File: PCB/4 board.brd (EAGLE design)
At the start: 82.6 x 57.5 mm, 17 parts, among them T1 2N2222, T2 2N2222, T3 2N2222

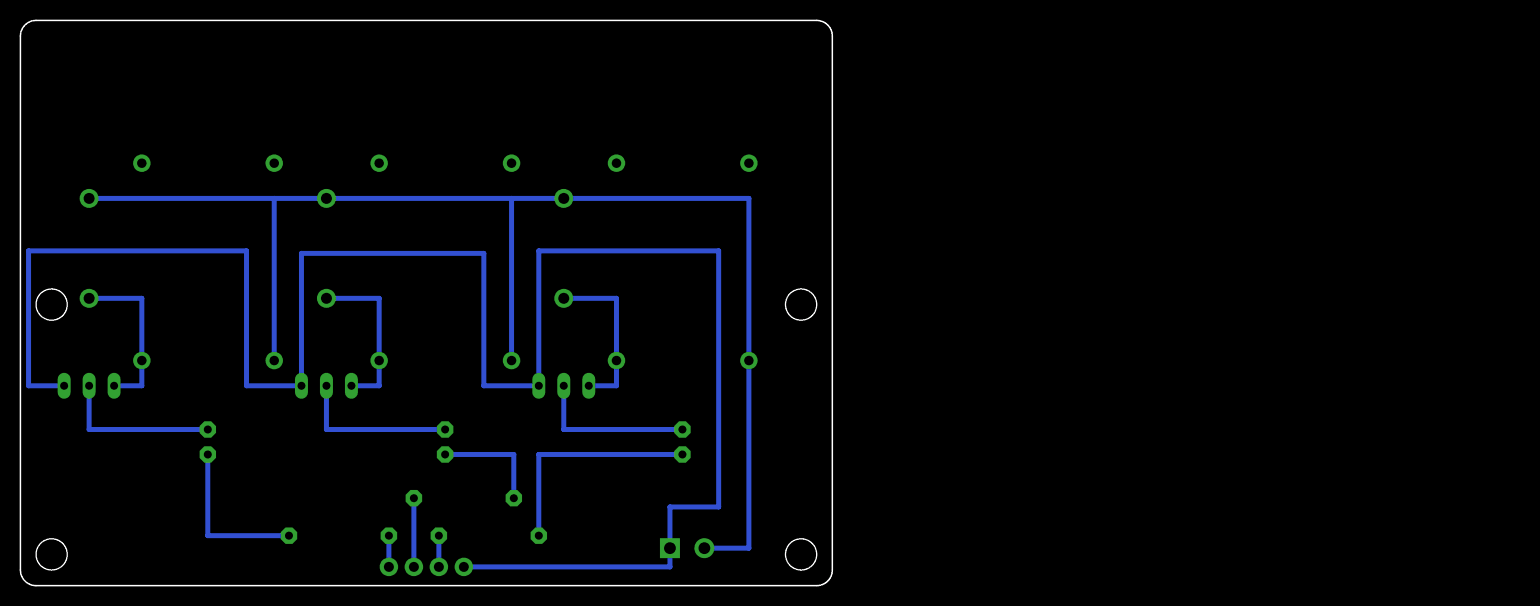
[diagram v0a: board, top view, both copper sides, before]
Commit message: 4 valve boards
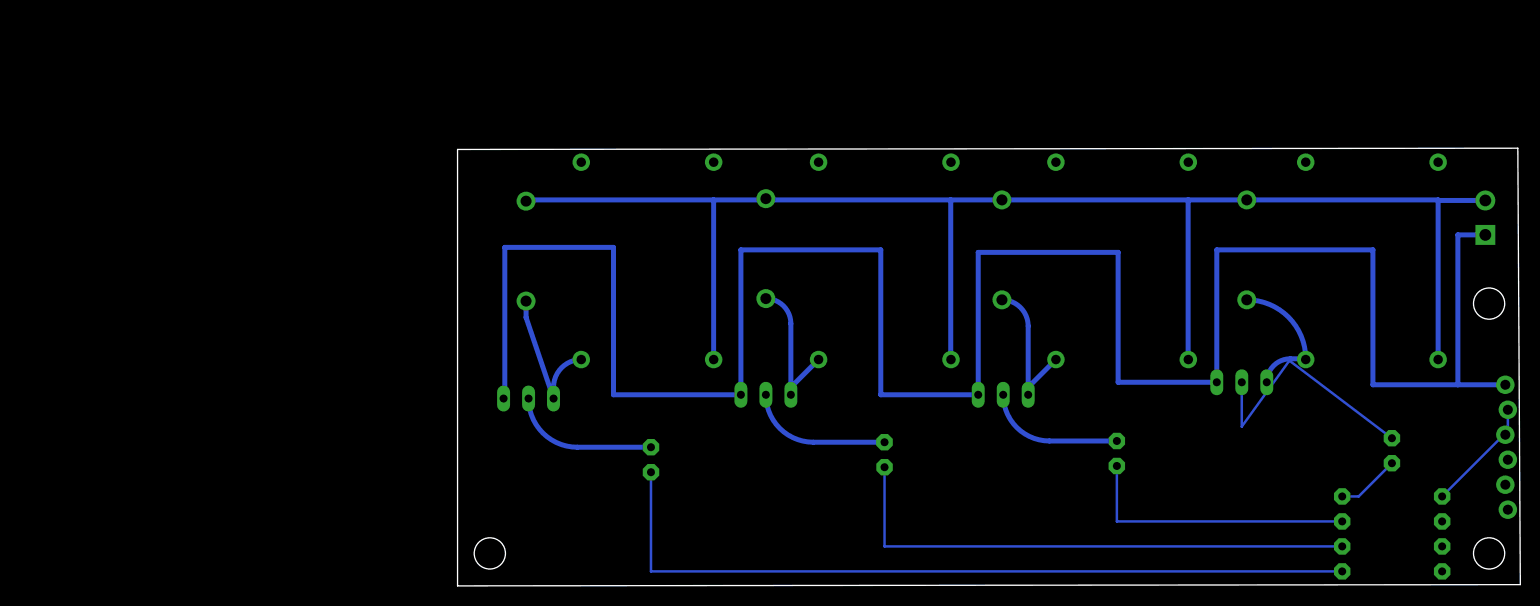
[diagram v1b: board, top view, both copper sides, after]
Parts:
- added D4: 1N4004, adafruit:DO41-10
- added LED4: (no value), adafruit:LED5MM
- added R4: (no value), adafruit:0207/10
- added T4: 2N2222, adafruit:TO92-EBC-OVAL
- added VALVE4: 4, local eagle library:VALVTEST2
- SV1: device SparkFun-Connectors:1X04 -> SparkFun-Connectors:1X06_LOCK
- moved SV1 113.9 mm to (106.8, 7.72), turned to 90 degrees
- moved R3 107.1 mm to (95.0, 3.99)
- moved R2 94.4 mm to (95.0, 6.53), turned to 0 degrees
- moved R1 91.9 mm to (95.0, 9.07), turned to 0 degrees
- moved J1 88.8 mm to (104.5, 35.7), turned to 90 degrees
- moved LED1 72.1 mm to (95.0, 13.7)
- moved U$1 70.1 mm to (100.6, 19.2)
- moved D1 69.4 mm to (80.2, 34.1)
- moved T1 68.9 mm to (79.7, 19.4)
- moved LED3 68.8 mm to (43.4, 13.3)
- moved T2 68.8 mm to (55.5, 18.1)
- moved T3 68.8 mm to (31.3, 18.1)
- moved U$2 68.8 mm to (75.2, 19.2)
- moved VALVE3 68.8 mm to (51.0, 19.2)
- moved D3 68.8 mm to (31.3, 34.3)
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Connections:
- new net N$12: LED4.A, R4.2
- new net N$4: D4.A, T4.C, VALVE4.PAD11
- new net N$43: R4.1, SV1.2
- new net N$45: SV1.1
- new net N$8: LED4.K, T4.B
- net 5V: now also D4.C, VALVE4.PAD10
- net GND: now also SV1.6, T4.E; no longer SV1.4
- net N$19: now also SV1.3; no longer SV1.1
- net N$30: now also SV1.5; no longer SV1.3
- net N$44: now also SV1.4; no longer SV1.2
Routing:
- net N$12: track 0.00 -> 80.4 mm
- net N$11: track 16.5 -> 54.6 mm
- net GND: track 199.9 -> 234.3 mm
- net 5V: track 140.1 -> 162.8 mm
- net N$7: track 11.4 -> 28.5 mm
- net N$3: track 22.9 -> 6.45 mm
- net N$4: track 0.00 -> 15.5 mm
- net N$8: track 0.00 -> 14.5 mm
- net N$2: track 16.5 -> 25.9 mm
- net N$30: track 3.17 -> 11.6 mm
- net N$44: track 6.99 -> 0.00 mm
- net N$1: track 17.1 -> 13.5 mm
- net N$19: track 3.17 -> 0.00 mm
- net N$6: track 16.5 -> 13.5 mm
- net N$10: track 16.5 -> 14.1 mm
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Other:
- board size 82.6 x 57.5 mm -> 108.1 x 44.5 mm
